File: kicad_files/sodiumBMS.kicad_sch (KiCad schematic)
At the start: 23 parts, among them J1 USB_C_Receptacle_PowerOnly_6P, U1 STM32F446RETx

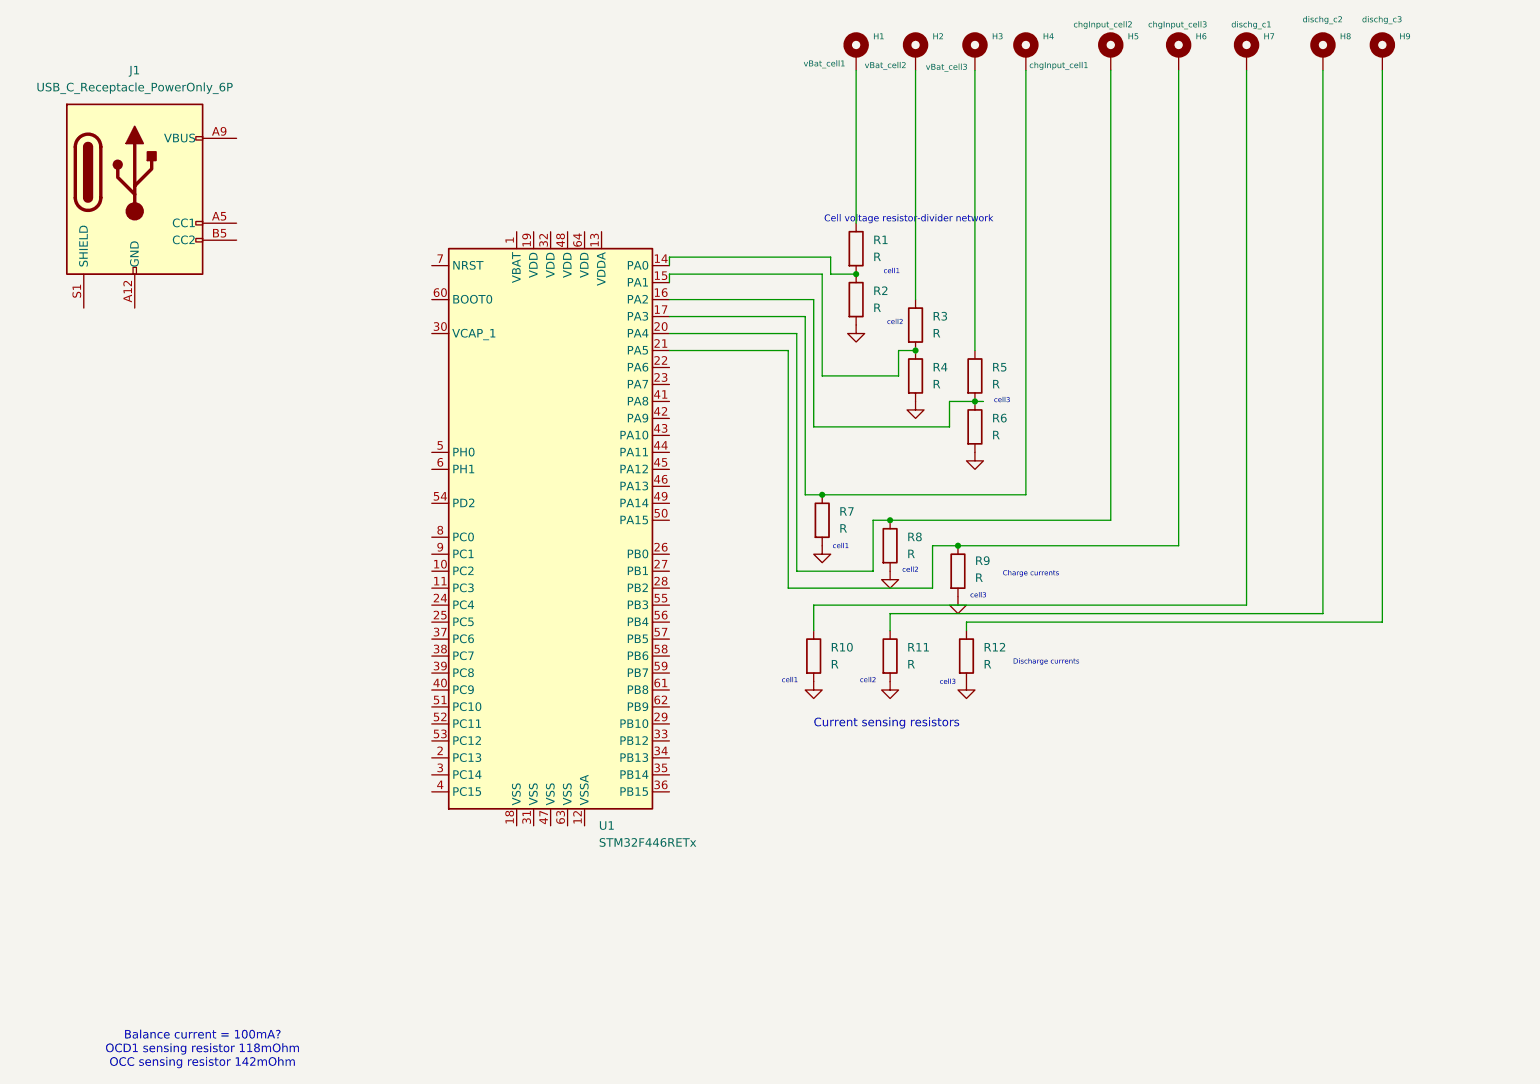
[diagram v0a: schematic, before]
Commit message: rearranged sch and added info about ICs
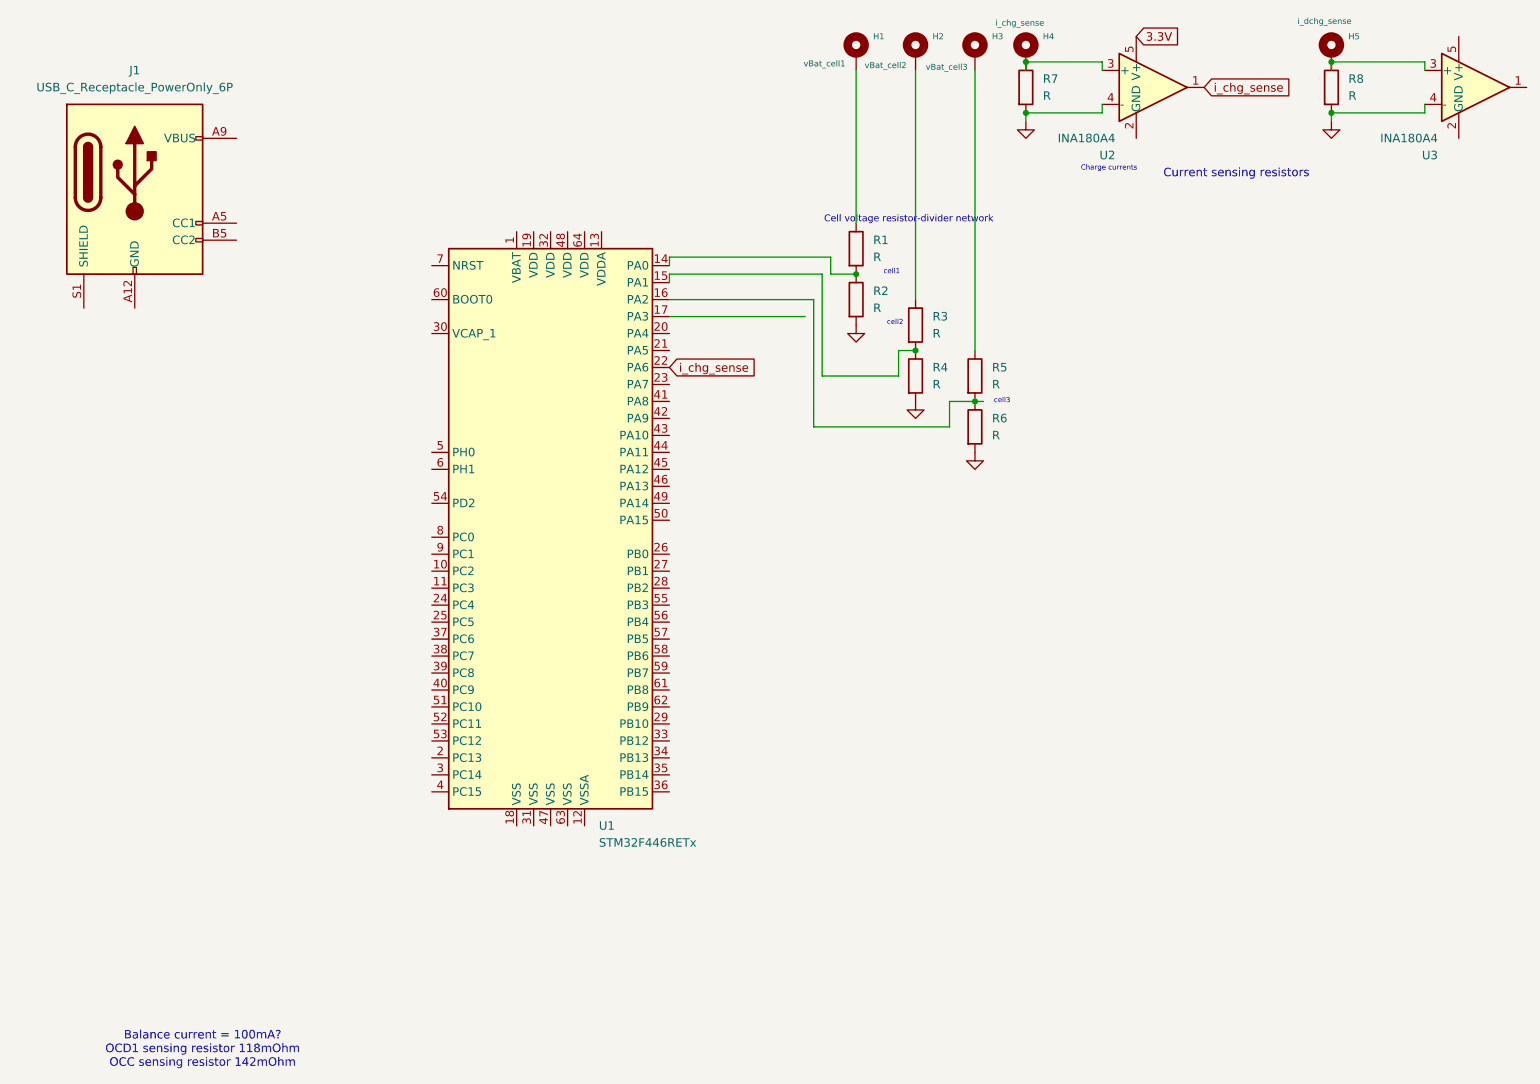
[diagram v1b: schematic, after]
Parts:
- removed H6: chgInput_cell3, symbol Mechanical:MountingHole_Pad
- removed H7: dischg_c1, symbol Mechanical:MountingHole_Pad
- removed H8: dischg_c2, symbol Mechanical:MountingHole_Pad
- removed H9: dischg_c3, symbol Mechanical:MountingHole_Pad
- removed R10, R11, R12, R9: R, symbol Device:R
- added U2, U3: INA180A4, Package_TO_SOT_SMD:SOT-23-5, symbol Amplifier_Current:INA180A4
- H4: value chgInput_cell1 -> i_chg_sense
- H5: value chgInput_cell2 -> i_dchg_sense
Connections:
- net GND: now also U2.4 (-), U3.4 (-)
- net at H5.1, R8.1: now also U3.3 (+); no longer U1.20 (PA4)
- net at H4.1, R7.1: now also U2.3 (+); no longer U1.17 (PA3)
- net i_chg_sense: now reaches U1.22 (PA6)
- net i_chg_sense: now also U2.1
- new net 3.3V: U2.5 (V+)
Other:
- note removed: "Discharge currents"
- moved on the sheet: H5, R7, R8
